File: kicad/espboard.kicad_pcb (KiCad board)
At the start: 2 copper layers, 48.3 x 40.6 mm, 14 parts, among them P1 CONN_PWR, P2 CONN_UART, P3 CONN_IO, SW1 SW_RST, SW2 SW_FLASH, U1 ESP-01v090, U2 LM1117-3.3

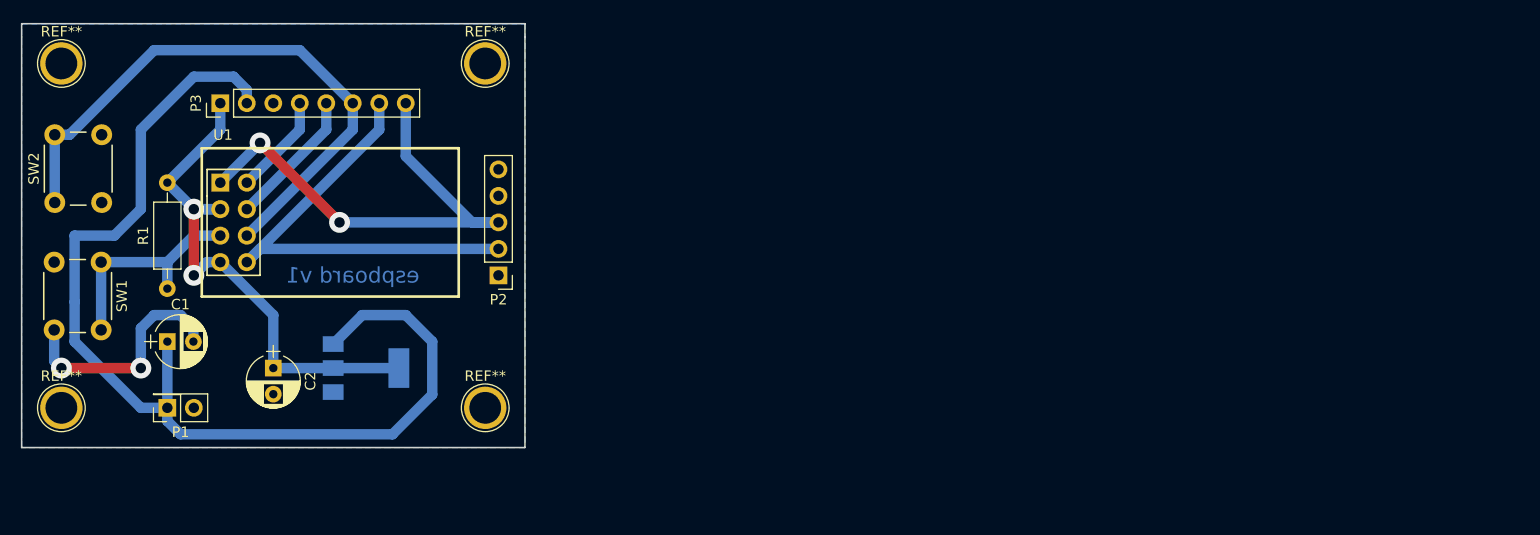
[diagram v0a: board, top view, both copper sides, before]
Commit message: v2
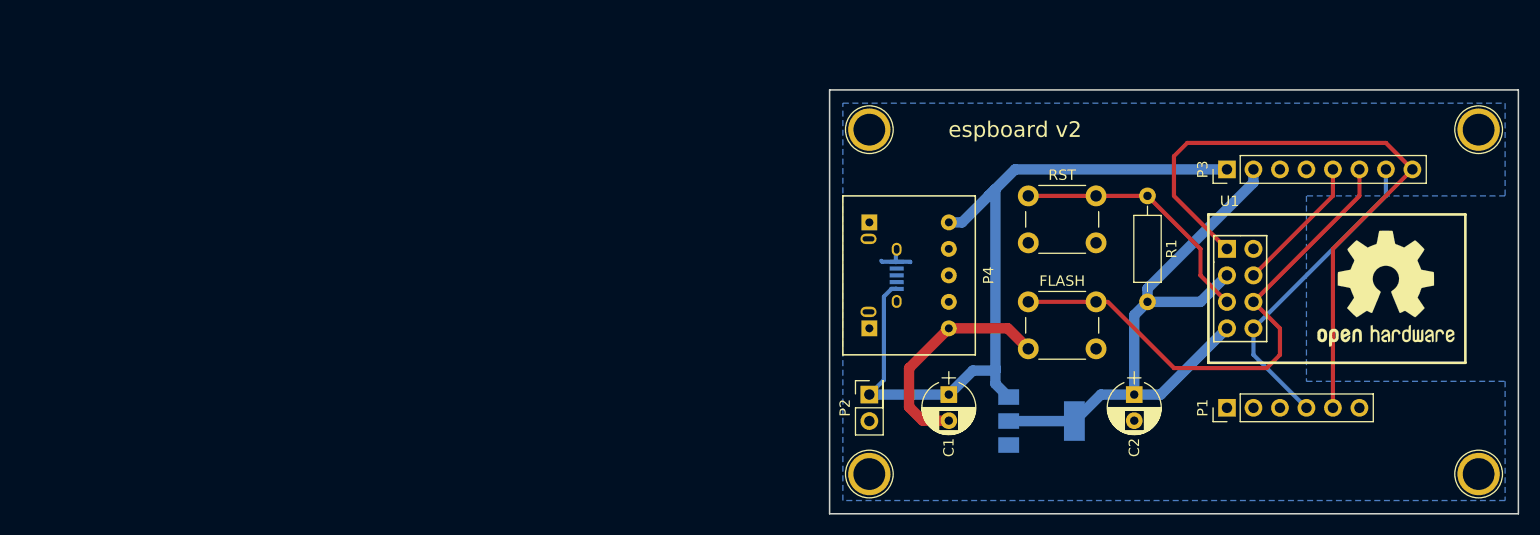
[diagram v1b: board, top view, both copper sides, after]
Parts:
- removed the REF** at (114.3, 76.2)
- removed the REF** at (114.3, 109.2)
- removed the REF** at (73.7, 109.2)
- removed the REF** at (73.7, 76.2)
- removed SW1: SW_RST, Buttons_Switches_THT:SW_PUSH_6mm
- removed SW2: SW_FLASH, Buttons_Switches_THT:SW_PUSH_6mm
- added FLASH: SW_FLASH, Buttons_Switches_THT:SW_PUSH_6mm, F.Cu at (166.4, 99.1)
- added J1: USB_OTG, Connectors:USB_Micro-B, B.Cu at (152.4, 96.5)
- added P4: usb_connector, usb_connector:usb_adapter, F.Cu at (158.8, 96.5)
- added REF**: 1pin, Connectors:1pin, F.Cu at (209.6, 82.5)
- added REF**: 1pin, Connectors:1pin, F.Cu at (209.6, 115.6)
- added REF**: 1pin, Connectors:1pin, F.Cu at (151.1, 115.6)
- added REF**: 1pin, Connectors:1pin, F.Cu at (151.1, 82.5)
- added REF***: OSHW-Logo2_14.6x12mm_SilkScreen, Symbols:OSHW-Logo2_14.6x12mm_SilkScreen, F.Cu at (200.7, 97.8)
- added RST: SW_RST, Buttons_Switches_THT:SW_PUSH_6mm, F.Cu at (166.4, 88.9)
- P1: value CONN_PWR -> ftdi; footprint Socket_Strips:Socket_Strip_Straight_2x01_Pitch2.54mm -> Pin_Headers:Pin_Header_Straight_1x06_Pitch2.54mm
- P2: value CONN_UART -> CONN_PWR; footprint Socket_Strips:Socket_Strip_Straight_1x05_Pitch2.54mm -> Socket_Strips:Socket_Strip_Straight_2x01_Pitch2.54mm
- moved P1 101.6 mm to (185.4, 109.2), turned to 90 degrees
- moved U1 96.7 mm to (185.4, 94.0)
- moved P3 96.7 mm to (185.4, 86.4)
- moved R1 94.4 mm to (177.8, 88.9), turned to 270 degrees
- moved C2 82.6 mm to (176.5, 108.0)
- moved C1 75.1 mm to (158.8, 108.0), turned to 270 degrees
- moved U2 65.0 mm to (167.6, 110.5)
- moved P2 37.4 mm to (151.1, 108.0), turned to 90 degrees
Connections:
- P1 pad 1: PWR_5V -> GND
- P1 pad 2: GND -> Net-(P1-Pad2)
- P2 pad 1: Net-(P2-Pad1) -> PWR_5V
- P2 pad 2: UART_TXD -> GND
- P3 pad 1: PWR_3V3 -> PWR_5V
- P3 pad 2: PWR_5V -> PWR_3V3
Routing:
- net PWR_5V: track 102.7 -> 75.1 mm
- net UART_TXD: track 45.2 -> 30.2 mm
- net UART_RXD: track 48.0 -> 61.4 mm, vias 2 -> 0
- net PWR_3V3: track 52.1 -> 59.6 mm, vias 2 -> 0
- net ESP_GPIO0: track 57.4 -> 50.3 mm
- net GND: track 32.5 -> 26.2 mm, vias 2 -> 0
- net Net-(R1-Pad1): track 21.4 -> 24.7 mm
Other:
- board size 48.3 x 40.6 mm -> 66 x 40.6 mm
- net class Default: trace_width 1 -> 0.4; via_dia 2 -> 0.4; via_drill 1 -> 0.3
- net class Power added: clearance 0.2, trace_width 1, via_dia 0.4, via_drill 0.3
- board text added: "espboard v2"
- board text removed: "espboard v1"
